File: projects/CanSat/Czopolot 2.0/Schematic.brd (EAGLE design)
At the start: 50.5 x 30.5 mm, 98 parts

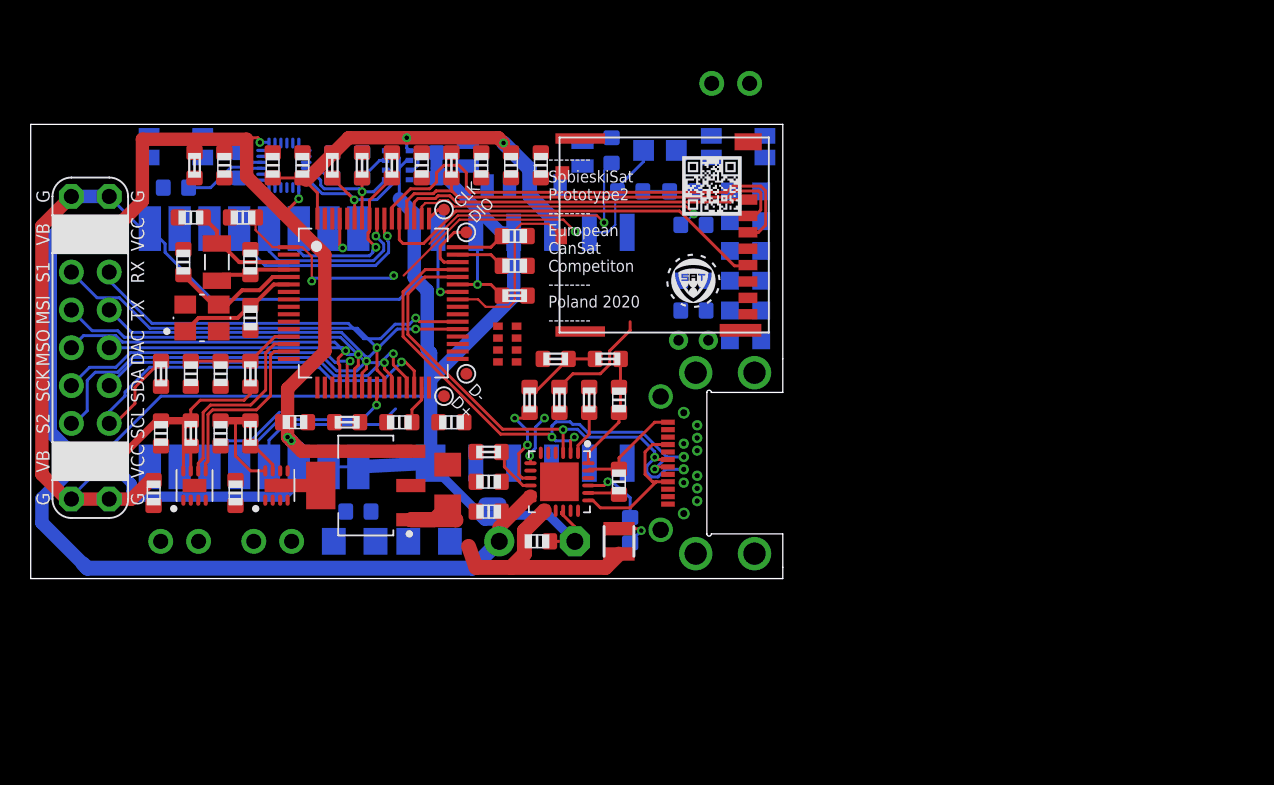
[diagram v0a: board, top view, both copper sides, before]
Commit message: Microcontroller and sensors done...
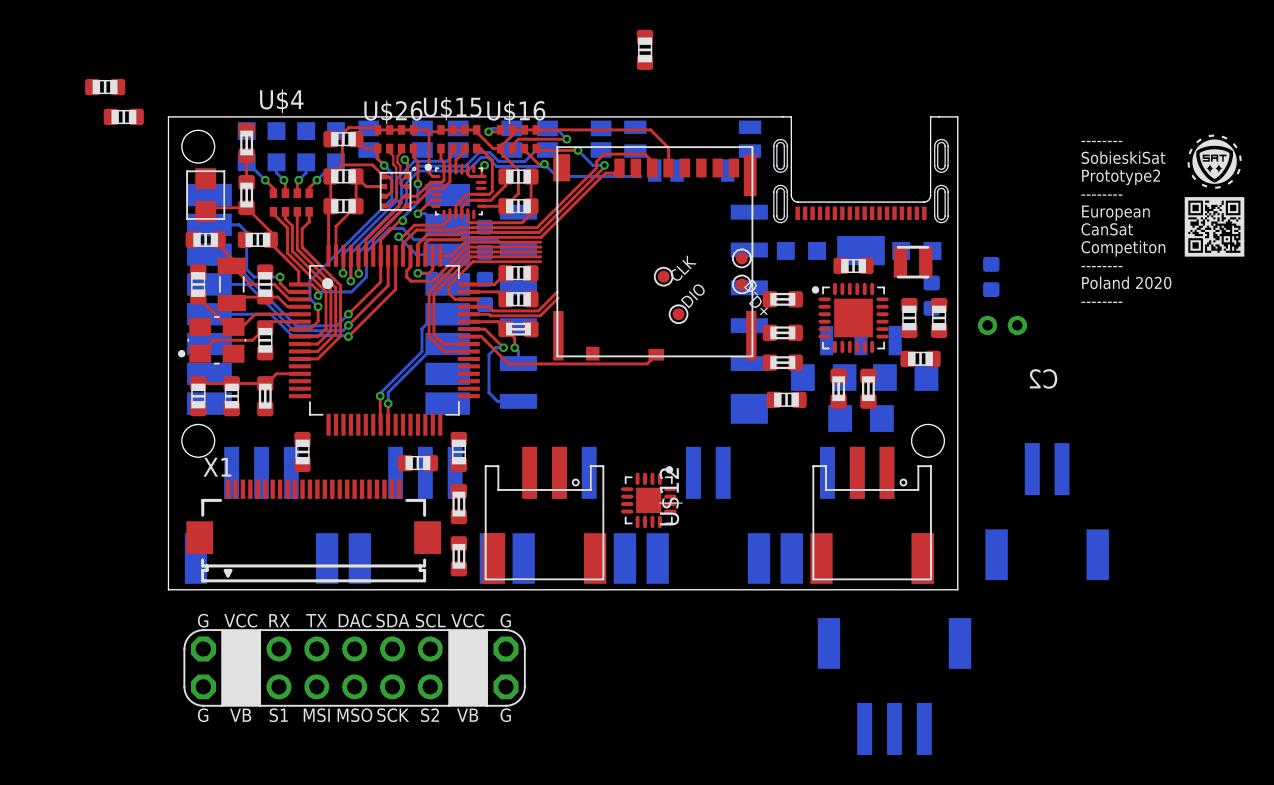
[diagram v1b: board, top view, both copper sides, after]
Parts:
- removed C40, C41: 100n, Unified:C0603
- removed C43, C44: 10u, Unified:C0603
- removed MOTL, MOTR: MOTOR, Unified:2X_JST
- removed R1, R13: 4.7k, Unified:R0603
- removed R12, R14, R3: 100k, Unified:R0603
- removed R40, R41, R7, R70, R71, R72, R8, R9: 10k, Unified:R0603
- removed R5: 560R, Unified:R0603
- removed RN1: 560R, SobieskiSat2:0603-ARC
- added BTN_USR1: PUSH-SWITCH, SobieskiSat2:SWITCH_SMD
- added U$12: TC78H653FTG, SobieskiSat2:QFN50P300X300X90-17T170N
- added U$13: MOTORJST_SMD, Unified:2X_JSTSMD_F
- added U$16, U$26: RESISTORARRAY, SobieskiSat2:0603-ARC
- added U$17, U$18: CONNECTOR_F_X2_JST_SMD, Unified:2X_JSTSMD_F
- added U$19, U$20, U$24, U$25: CONNECTOR_F_X3_JST_SMD, Unified:3X_JSTSMD_F
- added X1: FH12-24S-0.5SH, con-hirose:FH12-24S-0.5SH
- BAT_PACK: device SobieskiSat2:BAT_THT -> SobieskiSat2:2X_JSTSMD_F
- BTN_DFU: value PUSH-SWITCHDIP -> SLIDE-SWITCH; device SobieskiSat2:2X_JST -> SobieskiSat2:SLIDE-SWITCH
- U$14: value DRV8838 -> MOTORJST_SMD; device SobieskiSat2:SON50P200X200X80-9T90X160N -> Unified:2X_JSTSMD_F
- U$15: value DRV8838 -> RESISTORARRAY; device SobieskiSat2:SON50P200X200X80-9T90X160N -> SobieskiSat2:0603-ARC
- U$4: value SLIDE-SWITCH -> RESISTORARRAY; device SobieskiSat2:SLIDE-SWITCH -> SobieskiSat2:0603-ARC
- U$7: value USB-C -> USB2.0; device SobieskiSat2:USB-C -> SobieskiSat2:USB-C(2)
- moved U$23 35.9 mm to (67.8, 25.8)
- moved LM3940IMP 35.6 mm to (46.0, 18.8), flipped to the bottom, turned to 90 degrees
- moved U$14 34.6 mm to (35.8, 3.50), flipped to the bottom, turned to 180 degrees
- moved BAT_PACK 34.3 mm to (58.5, 3.75)
- moved U$22 33.9 mm to (67.8, 21.4)
- moved LEDA 33.6 mm to (4.75, 28.8), turned to 0 degrees
- moved C31 33.4 mm to (43.5, 13.2)
- moved C30 32.2 mm to (51.2, 17.2), turned to 90 degrees
- moved LEDB 31.9 mm to (6.75, 28.8), turned to 0 degrees
- moved C2 31.6 mm to (49.0, 13.2), flipped to the bottom, turned to 0 degrees
- moved C10 30.8 mm to (50.0, 14.5), turned to 0 degrees
- moved CBK 30.6 mm to (2.00, 25.5), flipped to the top, turned to 90 degrees
- moved LEDC 30.3 mm to (8.75, 28.8), turned to 0 degrees
- moved C23 30.2 mm to (46.0, 10.5)
- moved C21 29.6 mm to (54.8, 20.0)
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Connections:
- removed net EN_L: U$1.15, U$14.5
- removed net EN_R: U$1.17, U$15.5
- removed net GPIO_S1: U$1.26, U$11.6
- removed net GPIO_S2: U$1.27, U$11.10
- removed net N$23: C70.2, U$9.10
- removed net N$31: R40.1, U$14.7
- removed net N$34: MOTR.P$2, U$15.2
- removed net N$36: MOTR.P$1, U$15.3
- removed net N$40: R41.1, U$15.7
- removed net PH_L: U$1.14, U$14.6
- removed net PH_R: U$1.16, U$15.6
- new net EN_1: U$1.33
- new net EN_2: U$1.34
- new net EN_3: U$1.35
- new net EN_4: U$1.36
- new net MPU_REG: C70.2, U$9.10, U$9.14
- new net N$25: R0.1
- new net N$7: BTN_USR.P$1, BTN_USR.P$4, U$16.4
- new net PWM_1: U$1.27
- new net PWM_2: U$1.26
- new net PWM_3: U$1.37
- new net PWM_4: U$1.38
- net 43_D0: now also U$1.24; no longer U$1.25
- net 43_D1: now also U$1.25; no longer U$1.24
- net 43_MOSI: now also U$26.8; no longer R3.2
- net 43_NSS: now also U$1.2; no longer U$1.61
- net 43_RST: now also U$1.50; no longer R2.2, U$1.28
- net BAT: now also BAT_PACK.+; no longer BAT_PACK.P$2, C40.2, C43.2, U$14.1, U$15.1
- net BMP_SDI: now also U$26.7; no longer R9.1
- net BMP_SDO: now also U$26.6; no longer R8.2
- net DFU: now also U$16.7; no longer BTN_DFU.P$2, R12.1
- net GND: now also BAT_PACK.-, U$7.A1, U$7.A12, U$7.B1, U$7.B12, U$7.MID@1, U$7.MID@2, U$9.5; no longer BAT_PACK.P$1, BTN_USR.P$1, BTN_USR.P$4, C40.1, C41.1, C43.1, C44.1, R0.1, R12.2, R8.1, U$14.4, U$14.9, U$15.4, U$15.9, U$7.A$1, U$7.A$12, U$7.B$1, U$7.B$12, U$7.N$1, U$7.N$2, U$7.N$3, U$7.N$4, U$7.N$5, U$7.N$6
- net GPIO_RX: no longer U$1.38
- net GPIO_TX: no longer U$1.37
- net IMU_INT: no longer U$1.62
- net MPU_AD0: now also U$15.8, U$9.15; no longer R72.1
- net MPU_NCS: now also U$15.7; no longer R7.1
- net N$1: now also U$4.1; no longer RN1.7
- net N$10: no longer RN1.1
- net N$15: now also U$1.8, U$4.5; no longer R5.2, U$1.36
- net N$16: now also BTN_USR1.P$1, BTN_USR1.P$4, U$16.6; no longer BTN_USR.P$2, BTN_USR.P$3, R1.1
- net N$19: now also U$1.11, U$4.8; no longer RN1.4, U$1.35
- net N$2: now also U$4.2; no longer RN1.6
- net N$20: now also U$1.10, U$4.7; no longer RN1.3, U$1.34
- net N$26: now also U$1.9, U$4.6; no longer MOTL.P$1, U$14.3
- net N$28: now also BTN_USR1.P$2, BTN_USR1.P$3, U$1.61; no longer RN1.2, U$1.33
- net N$3: no longer RN1.8
- net N$37: now also U$4.3; no longer RN1.5
- net N$38: now also U$4.4; no longer R5.1
- net N$4: now also R2.2, U$1.28; no longer R1.2, U$1.50
- net N$5: now also BTN_USR.P$2, BTN_USR.P$3, U$1.62; no longer MOTL.P$2, U$14.2
- net NRST: now also U$26.5; no longer R13.1
- net SCL: now also U$15.6, U$9.3; no longer R71.1
- net SDA: now also U$15.5, U$9.2; no longer R70.1
- net SD_D3: now also U$16.8; no longer R14.2
- net USB_D+: now also U$7.A6, U$7.B6; no longer U$7.A$6, U$7.B$6
- net USB_D-: now also U$7.A7, U$7.B7; no longer U$7.A$7, U$7.B$7
- net USB_VBUS: now also U$7.A4, U$7.A9, U$7.B4, U$7.B9; no longer U$7.A$4, U$7.A$9, U$7.B$4, U$7.B$9
- net VCC: now also U$15.1, U$15.2, U$15.3, U$15.4, U$16.1, U$16.2, U$16.3, U$16.5, U$26.1, U$26.2, U$26.3, U$26.4; no longer BTN_DFU.P$1, C41.2, C44.2, LEDP.A, R13.2, R14.1, R3.1, R40.2, R41.2, R7.2, R70.2, R71.2, R72.2, R9.2, U$14.8, U$15.8
- net VSYS: now also LEDP.A
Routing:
- net GND: track 163.3 -> 23.3 mm, vias 0 -> 3
- net VCC: track 124.7 -> 59.8 mm, vias 6 -> 1
- net BAT: track 58.7 -> 0.00 mm
- net GPIO_SCL: track 30.8 -> 0.00 mm, vias 1 -> 0
- net USB_D+: track 35.8 -> 6.59 mm, vias 3 -> 0
- net USB_D-: track 33.3 -> 6.53 mm, vias 2 -> 0
- net GPIO_S2: track 26.5 -> 0.00 mm, vias 1 -> 0
- net GPIO_RX: track 26.3 -> 0.00 mm, vias 1 -> 0
- net GPIO_S1: track 25.5 -> 0.00 mm, vias 1 -> 0
- net GPIO_TX: track 25.5 -> 0.00 mm, vias 1 -> 0
- net GPIO_SDA: track 23.4 -> 0.00 mm, vias 1 -> 0
- net GPIO_MOSI: track 23.1 -> 0.00 mm, vias 1 -> 0
- net VSYS: track 22.7 -> 0.00 mm
- net GPIO_MISO: track 22.5 -> 0.00 mm, vias 1 -> 0
- net GPIO_SCK: track 21.8 -> 0.00 mm, vias 1 -> 0
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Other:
- board size 50.5 x 30.5 mm -> 53 x 31.8 mm
- board text removed: "X"
- board text removed: "Y"
- board text removed: "Z"
